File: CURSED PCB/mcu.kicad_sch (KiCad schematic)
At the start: 22 parts, among them U1 STM32G431KBT6, U3 MIC94090YC6, Y1 24MHz crystal

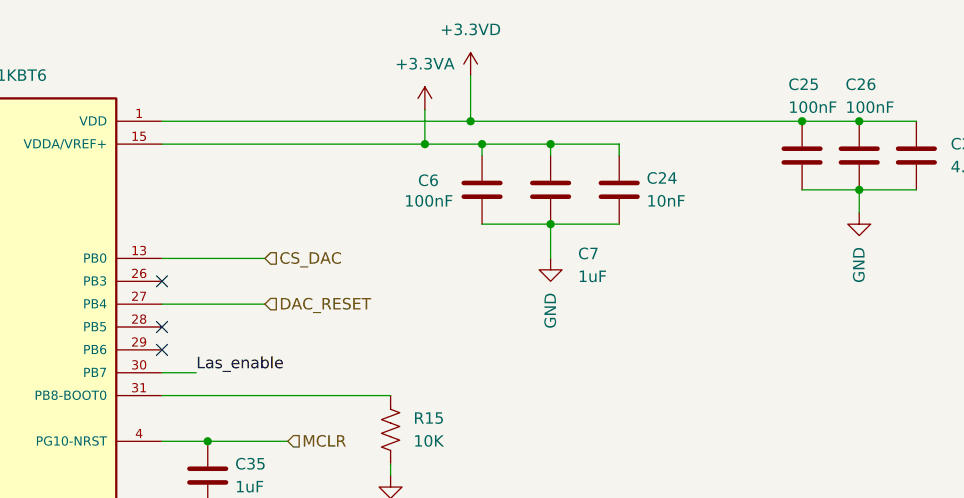
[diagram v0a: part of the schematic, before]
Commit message: forgot to commit
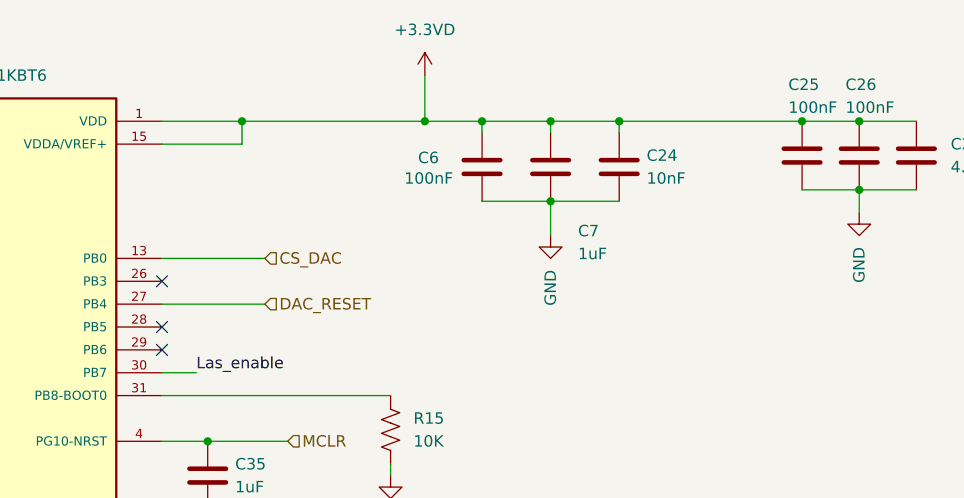
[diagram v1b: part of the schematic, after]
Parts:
- C2, C24, C25, C26, C27, C35, C5, C6, C7: footprint Capacitor_SMD:C_0805_2012Metric_Pad1.18x1.45mm_HandSolder -> Capacitor_SMD:C_0603_1608Metric_Pad1.08x0.95mm_HandSolder
- R1, R15, R2: footprint Resistor_SMD:R_0805_2012Metric_Pad1.20x1.40mm_HandSolder -> Resistor_SMD:R_0603_1608Metric_Pad0.98x0.95mm_HandSolder
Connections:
- net +3.3VA is gone; now on net +3.3VD: C24.2, C6.1, C7.2, U1.15 (VDDA/VREF+)
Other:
- moved on the sheet: C24, C6, C7
